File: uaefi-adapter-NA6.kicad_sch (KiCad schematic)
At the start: 2 parts, among them P1 178780-1

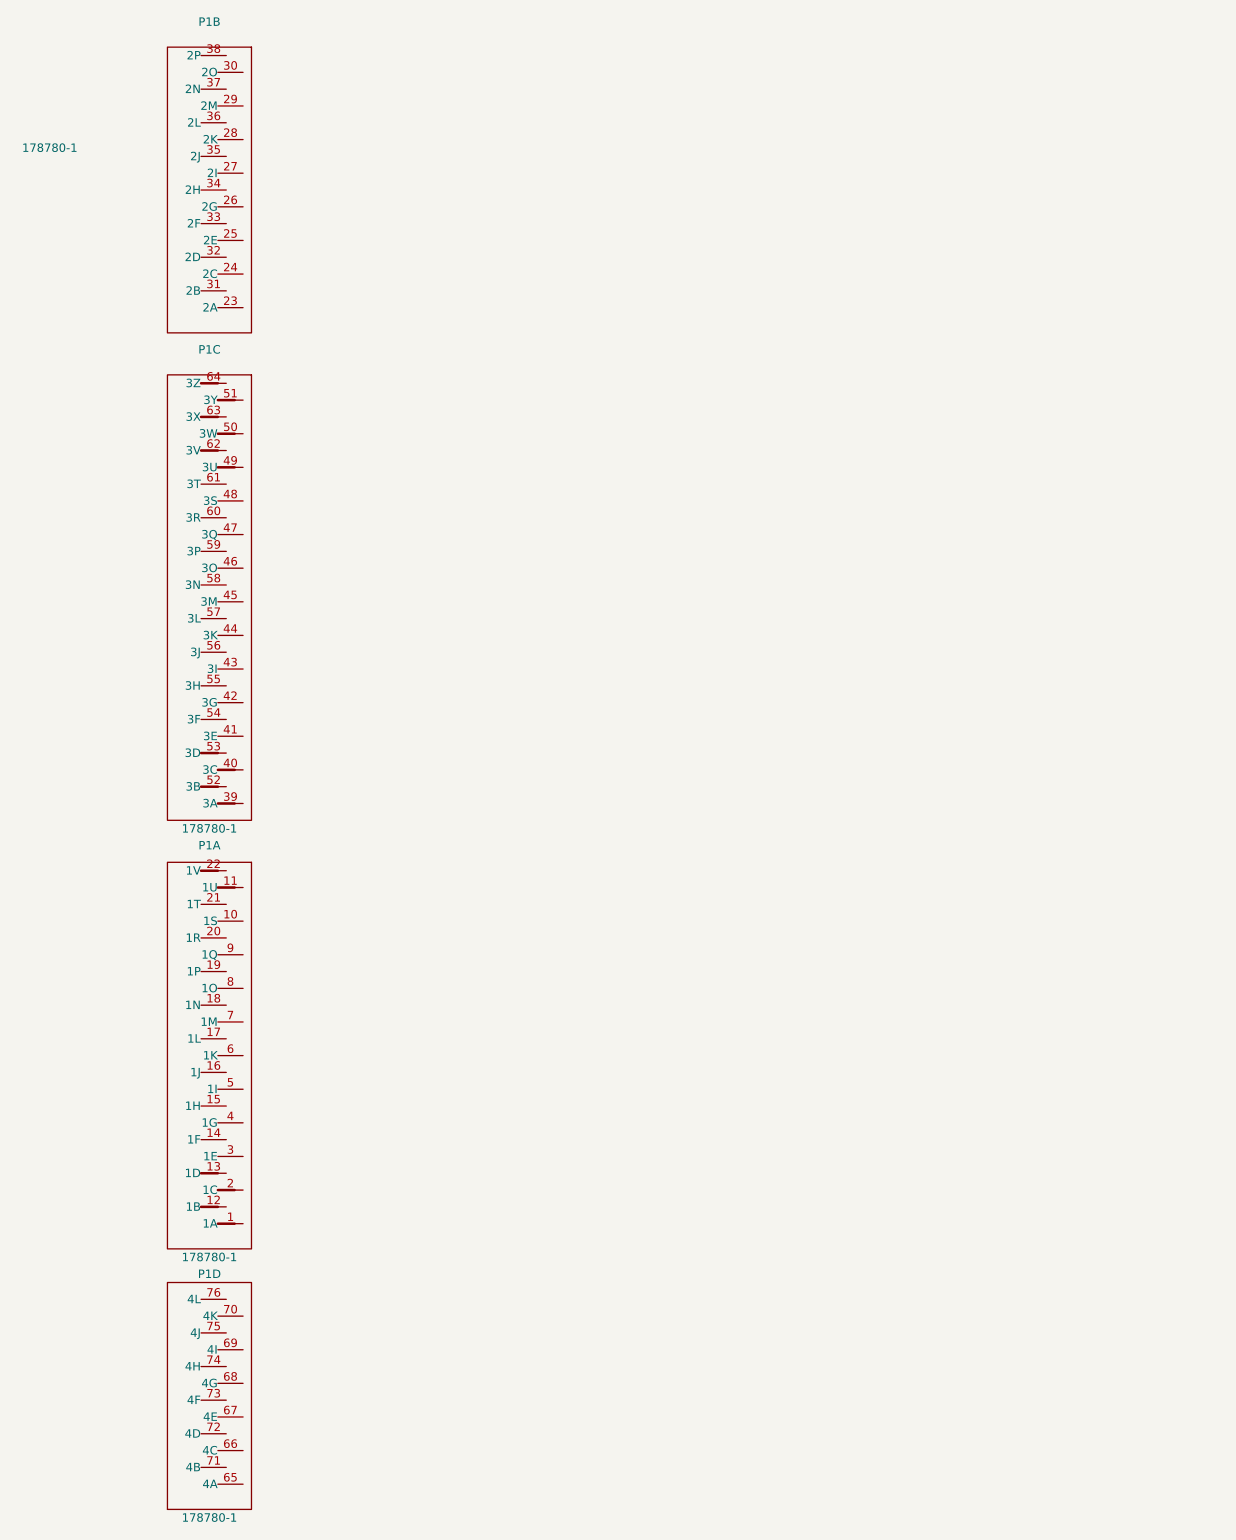
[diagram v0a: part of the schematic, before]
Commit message: upd
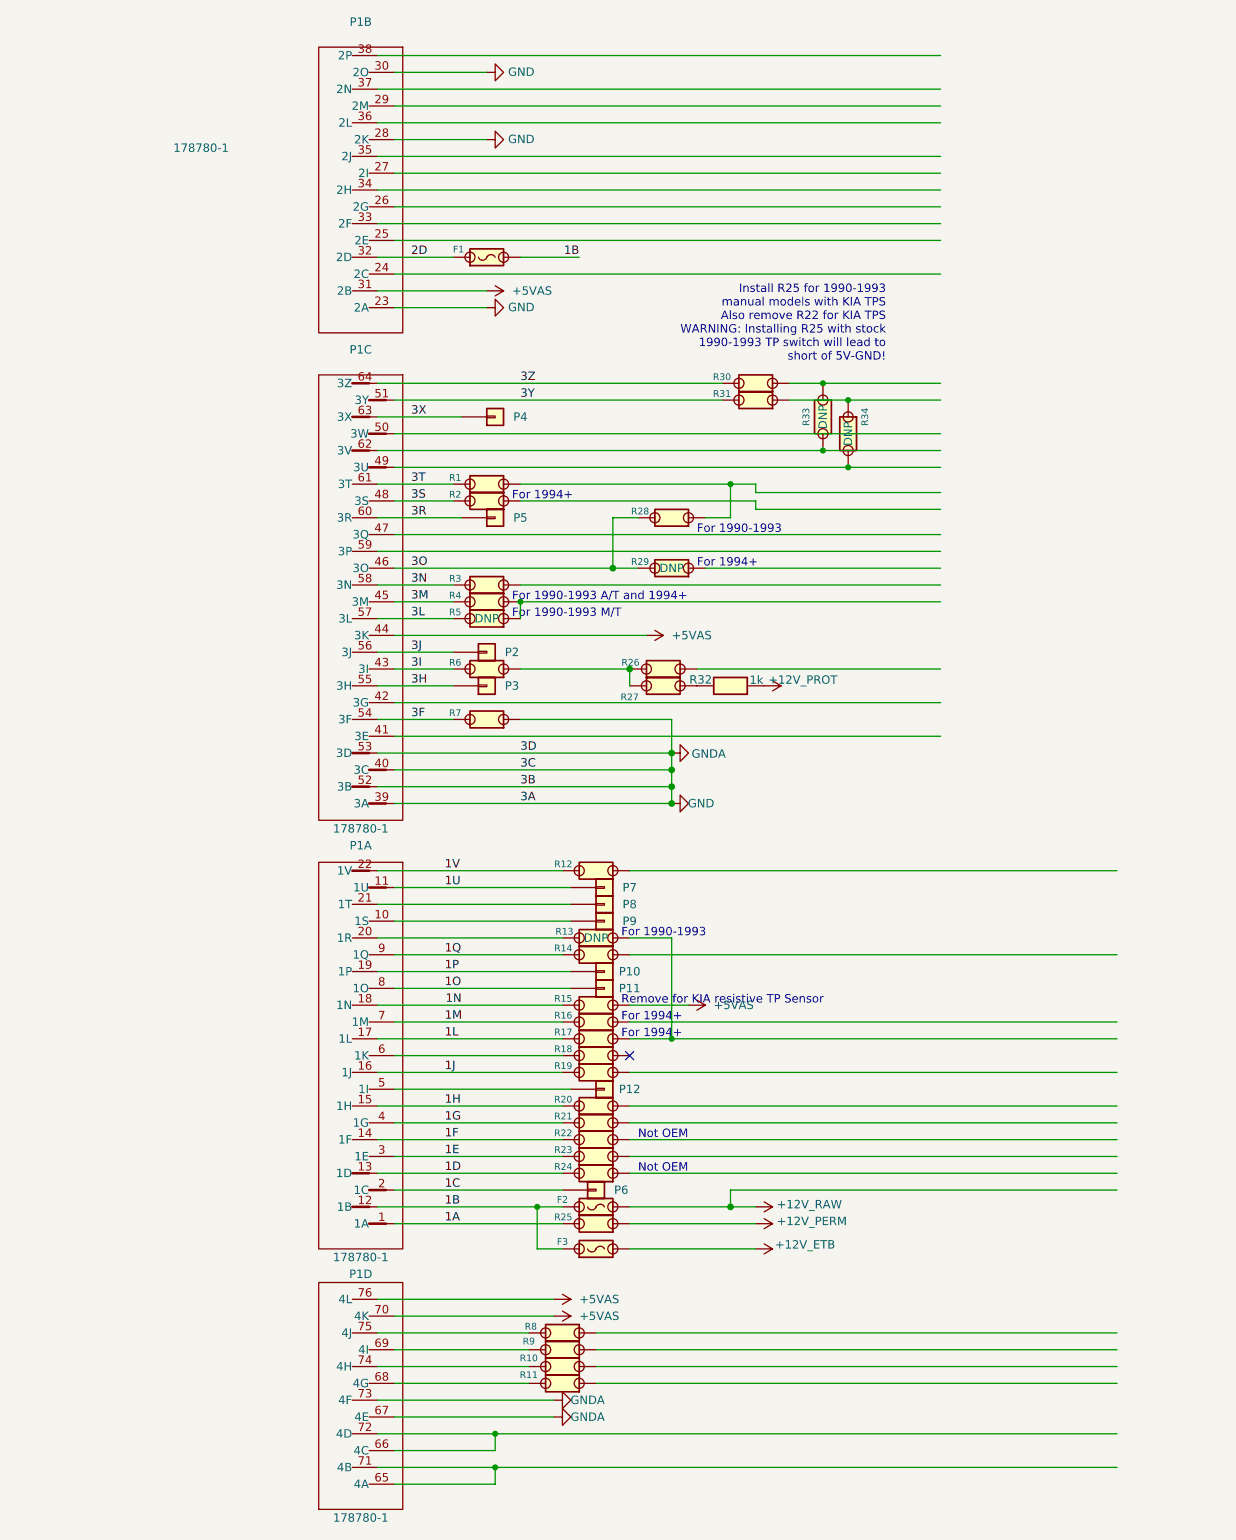
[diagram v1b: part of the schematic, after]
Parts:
- added F1, F2, F3: Fuse-Pad-Pad, hellen-one-common:PAD-1206-PAD, symbol hellen-one-common:Fuse-Pad-Pad
- added P10, P11, P12, P2, P3, P4, P5, P6, P7, P8, P9: Pad, hellen-one-common:PAD-TH, symbol hellen-one-common:Pad
- added R1, R10, R11, R12, R13, R14, R15, R16, R17, R18, R19, R2, R20, R21, R22, R23, R24, R25, R26, R27, R28, R29, R3, R30, R31, R33, R34, R4, R5, R6, R7, R8, R9: Jumper-Pad-Pad, hellen-one-common:PAD-0805-PAD, symbol hellen-one-common:Jumper-Pad-Pad
- added R32: 1k, hellen-one-common:R0603, symbol hellen-one-common:Res
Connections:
- net at P1.65 (4A): now also P1.71 (4B)
- net at P1.66 (4C): now also P1.72 (4D)
- net GND: now reaches P1.67 (4E)
- net GND: now also P1.23 (2A), P1.28 (2K), P1.30 (2O), P1.39 (3A), P1.40 (3C), P1.52 (3B), P1.53 (3D), P1.73 (4F), R7.1
- net at P1.68 (4G): now also R11.2
- net at P1.69 (4I): now also R9.2
- net +5VAS: now reaches P1.70 (4K)
- net +5VAS: now also P1.31 (2B), P1.44 (3K), P1.76 (4L), R15.1
- net at P1.74 (4H): now also R10.2
- net at P1.75 (4J): now also R8.2
- net 2D: now reaches P1.32 (2D)
- net 2D: now also F1.1
- net 3I: now reaches P1.43 (3I)
- net 3I: now also R6.2
- net 3M: now reaches P1.45 (3M)
- net 3M: now also R4.2
- net 3O: now reaches P1.46 (3O)
- net 3O: now also R28.2, R29.2
- net 3S: now reaches P1.48 (3S)
- net 3S: now also R2.2
- net at P1.49 (3U): now also R34.2
- net 3Y: now reaches P1.51 (3Y)
- net 3Y: now also R31.2
- net 3F: now reaches P1.54 (3F)
- net 3F: now also R7.2
- net 3H: now reaches P1.55 (3H)
- net 3H: now also P3.1 (Pin_1)
- net 3J: now reaches P1.56 (3J)
- net 3J: now also P2.1 (Pin_1)
- net 3L: now reaches P1.57 (3L)
- net 3L: now also R5.2
- net 3N: now reaches P1.58 (3N)
- net 3N: now also R3.2
- net 3R: now reaches P1.60 (3R)
- net 3R: now also P5.1 (Pin_1)
- net 3T: now reaches P1.61 (3T)
- net 3T: now also R1.2
- net at P1.62 (3V): now also R33.2
- net 3X: now reaches P1.63 (3X)
- net 3X: now also P4.1 (Pin_1)
- net 3Z: now reaches P1.64 (3Z)
- net 3Z: now also R30.2
- net 1A: now reaches P1.1 (1A)
- net 1A: now also R25.2
- net at P1.10 (1S): now also P9.1 (Pin_1)
- net 1U: now reaches P1.11 (1U)
- net 1U: now also P7.1 (Pin_1)
- net 1B: now reaches P1.12 (1B)
- net 1B: now also F1.2, F2.1, F3.1
- net 1D: now reaches P1.13 (1D)
- net 1D: now also R24.2
- net 1F: now reaches P1.14 (1F)
- net 1F: now also R22.2
- net 1H: now reaches P1.15 (1H)
- net 1H: now also R20.2
- net 1J: now reaches P1.16 (1J)
- net 1J: now also R19.2
- net 1L: now reaches P1.17 (1L)
- net 1L: now also R17.2
- net 1N: now reaches P1.18 (1N)
- net 1N: now also R15.2
- net 1P: now reaches P1.19 (1P)
- net 1P: now also P10.1 (Pin_1)
- net 1C: now reaches P1.2 (1C)
- net 1C: now also P6.1 (Pin_1)
- net at P1.20 (1R): now also R13.2
- net at P1.21 (1T): now also P8.1 (Pin_1)
- net 1V: now reaches P1.22 (1V)
- net 1V: now also R12.2
- net 1E: now reaches P1.3 (1E)
- net 1E: now also R23.2
- net 1G: now reaches P1.4 (1G)
- net 1G: now also R21.2
- net at P1.5 (1I): now also P12.1 (Pin_1)
- net at P1.6 (1K): now also R18.2
- net 1M: now reaches P1.7 (1M)
- net 1M: now also R16.2
- net 1O: now reaches P1.8 (1O)
- net 1O: now also P11.1 (Pin_1)
- net 1Q: now reaches P1.9 (1Q)
- net 1Q: now also R14.2
- new net: R13.1, R17.1
- new net: R30.1, R33.1
- new net: R1.1, R28.1
- new net: R26.2, R27.1, R6.1
- new net: R27.2, R32.2
- new net: R4.1, R5.1
- new net: R31.1, R34.1
- new net +12V_ETB: F3.2
- new net +12V_PERM: R25.1
- new net +12V_PROT: R32.1
- new net +12V_RAW: F2.2
- no-connect marks 0 -> 1
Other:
- note added: "For 1990-1993"
- note added: "For 1990-1993 A/T and 1994+"
- note added: "For 1990-1993 M/T"
- note added: "For 1994+"
- note added: "Install R25 for 1990-1993 manual models with KIA TPS Also remove R22 for KIA TPS WARNING: Installing R25 with stock 1990-1993 TP switch will lead to short of 5V-GND!"
- note added: "Not OEM"
- note added: "Remove for KIA resistive TP Sensor"
